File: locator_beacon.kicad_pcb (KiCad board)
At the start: 2 copper layers, 51 x 21.3 mm, 46 parts, among them J1 Conn_01x02, J2 Conn_01x02, J3 Conn_01x01, J4 OSHW logo, J5 Conn_01x02, J6 Conn_01x01, J7 Conn_01x01, J8 Conn_01x01, U1 DMHT6016LFJ-13, U13 Pico, U2 MIC2288, U3 MIC4606, U4 MIC2288

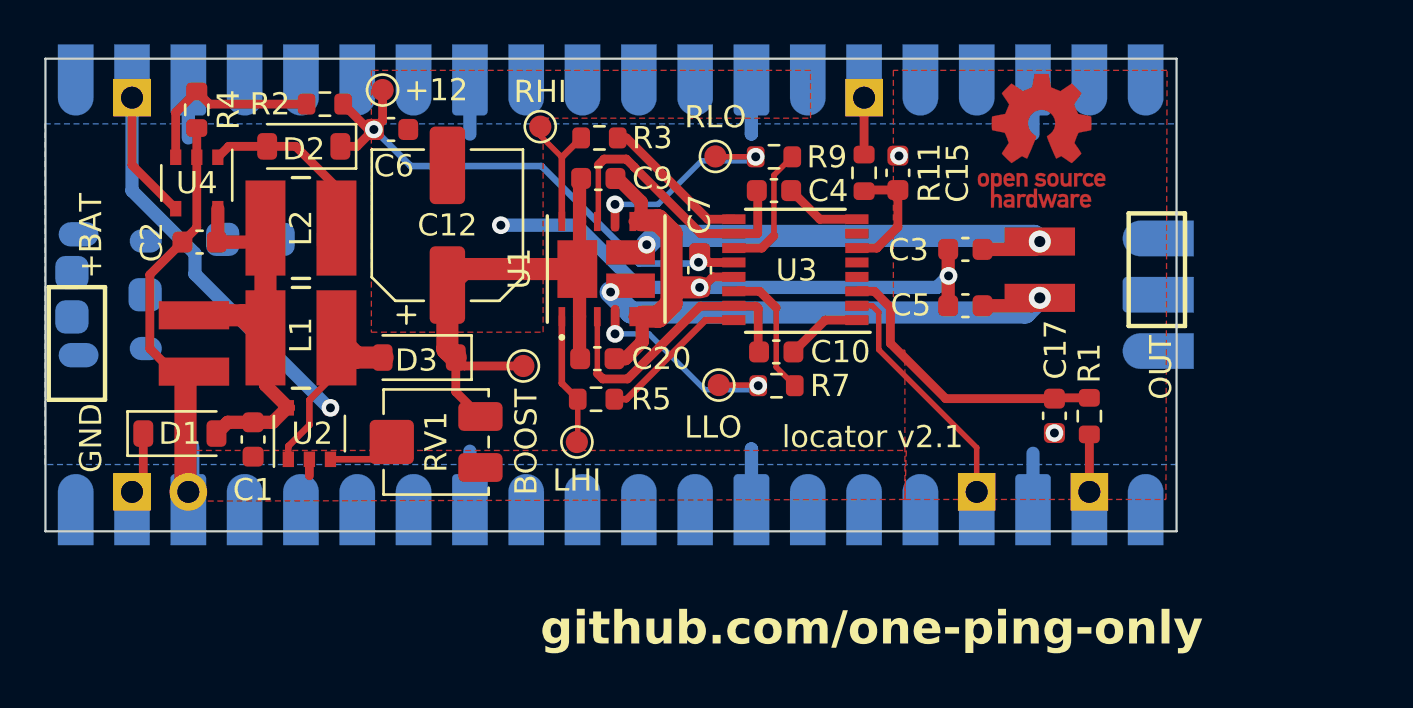
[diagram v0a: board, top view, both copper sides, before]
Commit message: 555 driver
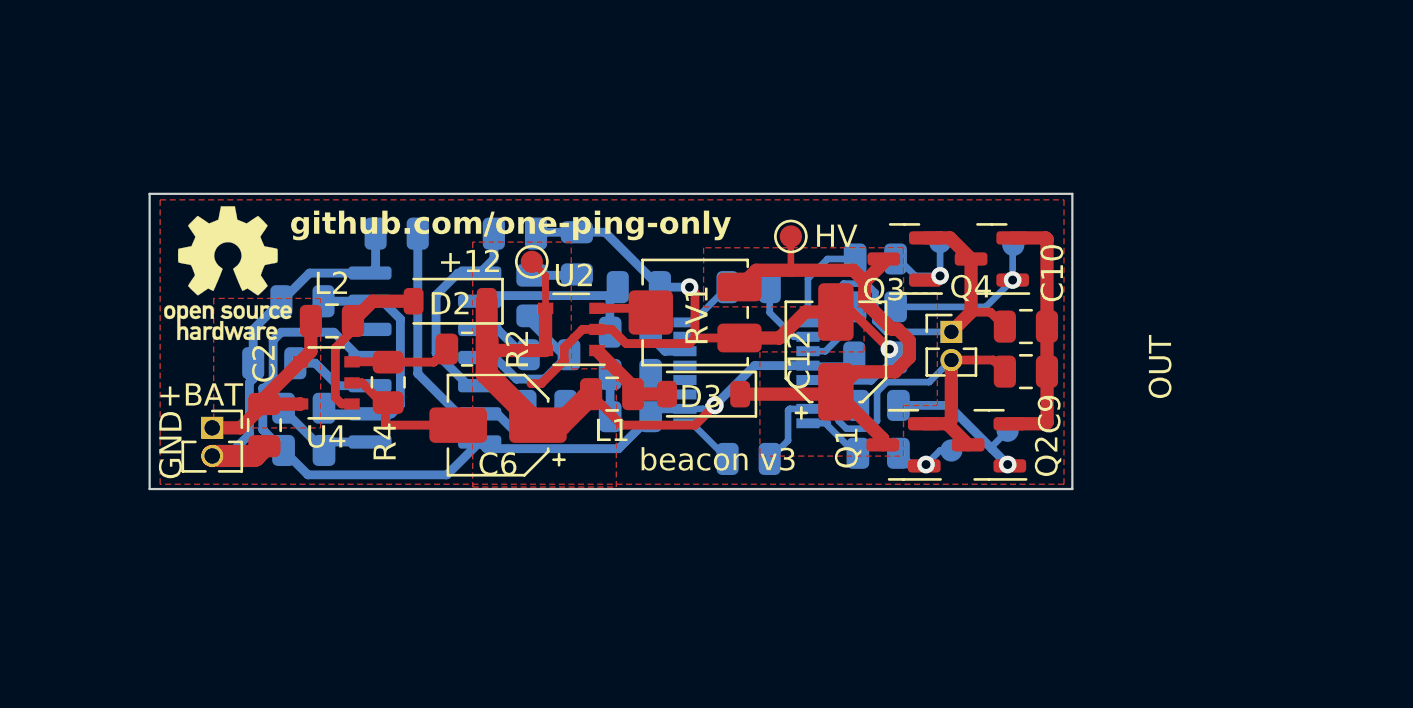
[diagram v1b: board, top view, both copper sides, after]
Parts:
- removed +12: +12, TestPoint:TestPoint_Pad_D1.0mm
- removed C15, C17: 1.5n, Capacitor_SMD:C_0603_1608Metric
- removed C20: 10u, Capacitor_SMD:C_0603_1608Metric
- removed D1: DSS16U, Diode_SMD:D_SOD-123
- removed J3, J6, J7, J8: Conn_01x01, Connector_PinHeader_2.54mm:PinHeader_1x01_P2.54mm_Vertical
- removed J5: Conn_01x02, Connector_PinHeader_2.54mm:PinHeader_1x02_P2.54mm_Vertical
- removed TP7: RHI, TestPoint:TestPoint_Pad_D1.0mm
- removed U13: Pico, custom:RPi_pico
- added C11: 10u, Capacitor_SMD:C_0805_2012Metric, B.Cu at (129.4, 78.7)
- added C13: 10u, Capacitor_SMD:C_0805_2012Metric, B.Cu at (141.7, 76.6)
- added C14: 1n, Capacitor_SMD:C_0805_2012Metric, B.Cu at (138.9, 75.7)
- added C8: 10n, Capacitor_SMD:C_0805_2012Metric, B.Cu at (128.1, 81.5)
- added Q1: DMN6140L, Package_TO_SOT_SMD:SOT-23, F.Cu at (156.5, 85.2)
- added Q2: DMN6140L, Package_TO_SOT_SMD:SOT-23, F.Cu at (160.3, 85.2)
- added Q3: DMN6140L, Package_TO_SOT_SMD:SOT-23, F.Cu at (156.5, 76.8)
- added Q4: DMN6140L, Package_TO_SOT_SMD:SOT-23, F.Cu at (160.4, 76.8)
- added R10: 500, Resistor_SMD:R_0805_2012Metric, B.Cu at (140.5, 81.2)
- added R12: 500, Resistor_SMD:R_0805_2012Metric, B.Cu at (139.7, 78.5)
- added R13: 8.2k, Resistor_SMD:R_0805_2012Metric, B.Cu at (144.1, 83.9)
- added R14: 68k, Resistor_SMD:R_0805_2012Metric, B.Cu at (140.3, 83.4)
- added R6: 10k, Resistor_SMD:R_0805_2012Metric, B.Cu at (129.4, 85.5)
- added R8: 100, Resistor_SMD:R_0805_2012Metric, B.Cu at (129.4, 83.6)
- added TP3: HV, TestPoint:TestPoint_Pad_D1.0mm, F.Cu at (151.4, 75.8)
- added TP5: RHI, TestPoint:TestPoint_Pad_D1.0mm, B.Cu at (158.1, 76.1)
- C1: value C -> 1.5n; footprint Capacitor_SMD:C_0603_1608Metric -> Capacitor_SMD:C_0805_2012Metric; moved to B.Cu
- C10, C9: value 10u -> 220n; footprint Capacitor_SMD:C_0603_1608Metric -> Capacitor_SMD:C_0805_2012Metric
- C12: footprint Capacitor_SMD:CP_Elec_6.3x7.7 -> Capacitor_SMD:CP_Elec_4x3.9
- C2: footprint Capacitor_SMD:C_0603_1608Metric -> Capacitor_SMD:C_0805_2012Metric
- C3: value 220n -> 1.5n; footprint Capacitor_SMD:C_0603_1608Metric -> Capacitor_SMD:C_0805_2012Metric; moved to B.Cu
- C4, C7: footprint Capacitor_SMD:C_0603_1608Metric -> Capacitor_SMD:C_0805_2012Metric; moved to B.Cu
- C5: value 220n -> 10u; footprint Capacitor_SMD:C_0603_1608Metric -> Capacitor_SMD:C_0805_2012Metric; moved to B.Cu
- C6: footprint Capacitor_SMD:C_0603_1608Metric -> Capacitor_SMD:CP_Elec_4x3.9
- J1: value Conn_01x02 -> Conn_01x02_Pin; footprint custom:SAMTEC_TSM-102-01-L-SH -> Connector_PinSocket_1.27mm:PinSocket_1x02_P1.27mm_Vertical
- J2: value Conn_01x02 -> Conn_01x02_Pin; footprint custom:SAMTEC_TSM-102-01-L-SH -> Connector_PinHeader_1.27mm:PinHeader_1x02_P1.27mm_Vertical
- J4: footprint Symbol:OSHW-Logo_5.7x6mm_Copper -> Symbol:OSHW-Logo_5.7x6mm_SilkScreen
- L1, L2: footprint custom:IND_357100_WRE -> Capacitor_SMD:C_0805_2012Metric
- R1, R11, R3, R5, R7, R9: footprint Resistor_SMD:R_0603_1608Metric -> Resistor_SMD:R_0805_2012Metric; moved to B.Cu
- R2, R4: footprint Resistor_SMD:R_0603_1608Metric -> Resistor_SMD:R_0805_2012Metric
- TP1: value BOOST -> +12
- TP2, TP4, TP6: moved to B.Cu
- U1: value DMHT6016LFJ-13 -> MIC4606; footprint custom:V-DFN5045-12_DIO -> Package_SO:TSSOP-16-1EP_4.4x5mm_P0.65mm; moved to B.Cu
- U3: value MIC4606 -> LM556; footprint Package_SO:TSSOP-16-1EP_4.4x5mm_P0.65mm -> Package_SO:SO-14_3.9x8.65mm_P1.27mm; moved to B.Cu
- moved J1 43.2 mm to (125.3, 84.4), turned to 0 degrees
- moved J2 39.4 mm to (158.6, 80.1), turned to 0 degrees
- moved J4 37.2 mm to (126.0, 77.5)
- moved C3 25.7 mm to (133.6, 75.7)
- moved C9 21.2 mm to (162.0, 81.9)
- moved R1 20.8 mm to (144.1, 82.0), turned to 180 degrees
- moved C1 18.7 mm to (144.5, 78.1), turned to 0 degrees
- moved C12 18.4 mm to (153.4, 81.0)
- moved U3 17.2 mm to (134.9, 81.3), turned to 0 degrees
- moved TP2 16.9 mm to (158.6, 85.5)
- moved R4 15.0 mm to (133.2, 82.4)
- moved L1 14.3 mm to (143.3, 82.9)
- moved C6 14.2 mm to (138.2, 84.3), turned to 180 degrees
- moved TP6 14.0 mm to (161.4, 76.2)
- moved TP4 13.2 mm to (161.2, 84.6)
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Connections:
- C1 pad 1: +BATT -> /PWM_A
- C10 pad 1: Net-(U3-BHB) -> /OUT_B
- C10 pad 2: /amplifier/OUT_A -> GND
- C12 pad 1: V_{boost} -> /V_{HV}
- C3 pad 1: /amplifier/OUT_B -> /PWM_B
- C4 pad 1: Net-(U3-AHB) -> +12V
- C4 pad 2: /amplifier/OUT_B -> GND
- C5 pad 1: /amplifier/OUT_A -> Net-(U1-BHB)
- C5 pad 2: GND -> /OUT_A
- C7 pad 1: +12V -> Net-(U1-AHB)
- C7 pad 2: GND -> /OUT_B
- C9 pad 1: V_{boost} -> /OUT_A
- D3 pad 1: V_{boost} -> /V_{HV}
- L1 pad 1: +BATT -> +12V
- R1 pad 1: Net-(U3-BPWM) -> Net-(U1-BPWM)
- R1 pad 2: /amplifier/SIG_IN -> /PWM_B
- R11 pad 1: Net-(U3-APWM) -> /R_LO
- R11 pad 2: /amplifier/~{SIG_IN} -> Net-(U1-ALO)
- R3 pad 1: /amplifier/R_HI -> Net-(U1-APWM)
- R3 pad 2: Net-(U3-AHO) -> /PWM_A
- R5 pad 1: /amplifier/L_HI -> /L_HI
- R5 pad 2: Net-(U3-BHO) -> Net-(U1-BHO)
- R7 pad 1: /amplifier/L_LO -> /L_LO
- R7 pad 2: Net-(U3-BLO) -> Net-(U1-BLO)
- R9 pad 1: /amplifier/R_LO -> /R_HI
- R9 pad 2: Net-(U3-ALO) -> Net-(U1-AHO)
- RV1 pad 1: V_{boost} -> /V_{HV}
- TP1 pad 1: V_{boost} -> +12V
- TP2 pad 1: /amplifier/L_HI -> /L_HI
- TP4 pad 1: /amplifier/L_LO -> /L_LO
- TP6 pad 1: /amplifier/R_LO -> /R_LO
- U1 pad 1: /amplifier/L_HI -> Net-(U1-BHB)
- U1 pad 10: /amplifier/OUT_B -> /OUT_B
- U1 pad 11: V_{boost} -> Net-(U1-ALO)
- U1 pad 12: /amplifier/R_HI -> +12V
- U1 pad 13: V_{boost} -> GND
- U1 pad 14: /amplifier/OUT_A -> Net-(U1-BLO)
- U1 pad 15: /amplifier/OUT_B -> /OUT_A
- U1 pad 2: V_{boost} -> +12V
- U1 pad 3: /amplifier/OUT_A -> Net-(U1-BPWM)
- U1 pad 4: /amplifier/L_LO -> unconnected-(U1-NC-Pad4)
- U1 pad 5: GND -> unconnected-(U1-NC-Pad5)
- U1 pad 6: GND -> Net-(U1-APWM)
- U1 pad 7: GND -> unconnected-(U1-NC-Pad7)
- U1 pad 8: GND -> Net-(U1-AHB)
- U1 pad 9: /amplifier/R_LO -> Net-(U1-AHO)
- U2 pad 4: /power/EN -> +12V
- U2 pad 5: +BATT -> +12V
- U3 pad 1: Net-(U3-BHB) -> Net-(U3A-DIS)
- U3 pad 10: /amplifier/OUT_B -> /PULSE_START
- U3 pad 11: Net-(U3-ALO) -> Net-(U3B-CV)
- U3 pad 12: +12V -> /A
- U3 pad 13: GND -> /PWM_B
- U3 pad 14: Net-(U3-BLO) -> +12V
- U3 pad 2: /amplifier/EN -> /B
- U3 pad 3: Net-(U3-BPWM) -> Net-(U3A-CV)
- U3 pad 4: unconnected-(U3-NC-Pad4) -> +12V
- U3 pad 5: unconnected-(U3-NC-Pad5) -> /PULSE_START
- U3 pad 6: Net-(U3-APWM) -> /B
- U3 pad 7: unconnected-(U3-NC-Pad7) -> GND
- U3 pad 8: Net-(U3-AHB) -> /A
- U3 pad 9: Net-(U3-AHO) -> /PWM_A
- U4 pad 4: /power/EN -> +BATT
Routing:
- net +12V: track 25.0 -> 63.6 mm, vias 2 -> 1
- net /amplifier/OUT_A: track 36.0 -> 0.00 mm, vias 2 -> 0
- net /amplifier/OUT_B: track 33.6 -> 0.00 mm, vias 2 -> 0
- net /V_{HV}: track 0.00 -> 24.9 mm
- net V_{boost}: track 23.8 -> 0.00 mm
- net /power/EN: track 23.6 -> 0.00 mm, vias 1 -> 0
- net /OUT_B: track 0.00 -> 21.3 mm
- net /OUT_A: track 0.00 -> 20.6 mm
- net /PWM_B: track 0.00 -> 19.0 mm
- net Net-(U3-BPWM): track 13.5 -> 0.00 mm
- net /A: track 0.00 -> 12.0 mm
- net /B: track 0.00 -> 11.4 mm
- net /amplifier/EN: track 11.0 -> 0.00 mm
- net +BATT: track 19.9 -> 9.05 mm
- net /amplifier/L_LO: track 10.5 -> 0.00 mm, vias 2 -> 0
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- added copper zone on F.Cu, net +12V
- added copper zone on F.Cu, net +BATT
- added copper zone on F.Cu, net /V_{HV}
- removed copper zone on B.Cu, net GND
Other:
- board size 51 x 21.3 mm -> 41.6 x 13.3 mm
- board text added: "beacon v3"
- board text removed: "locator v2.1"
